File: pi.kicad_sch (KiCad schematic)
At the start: 5 parts, among them J5 2-1734839-0, J6 2-1734839-0, U15 MCP23008-E/ML

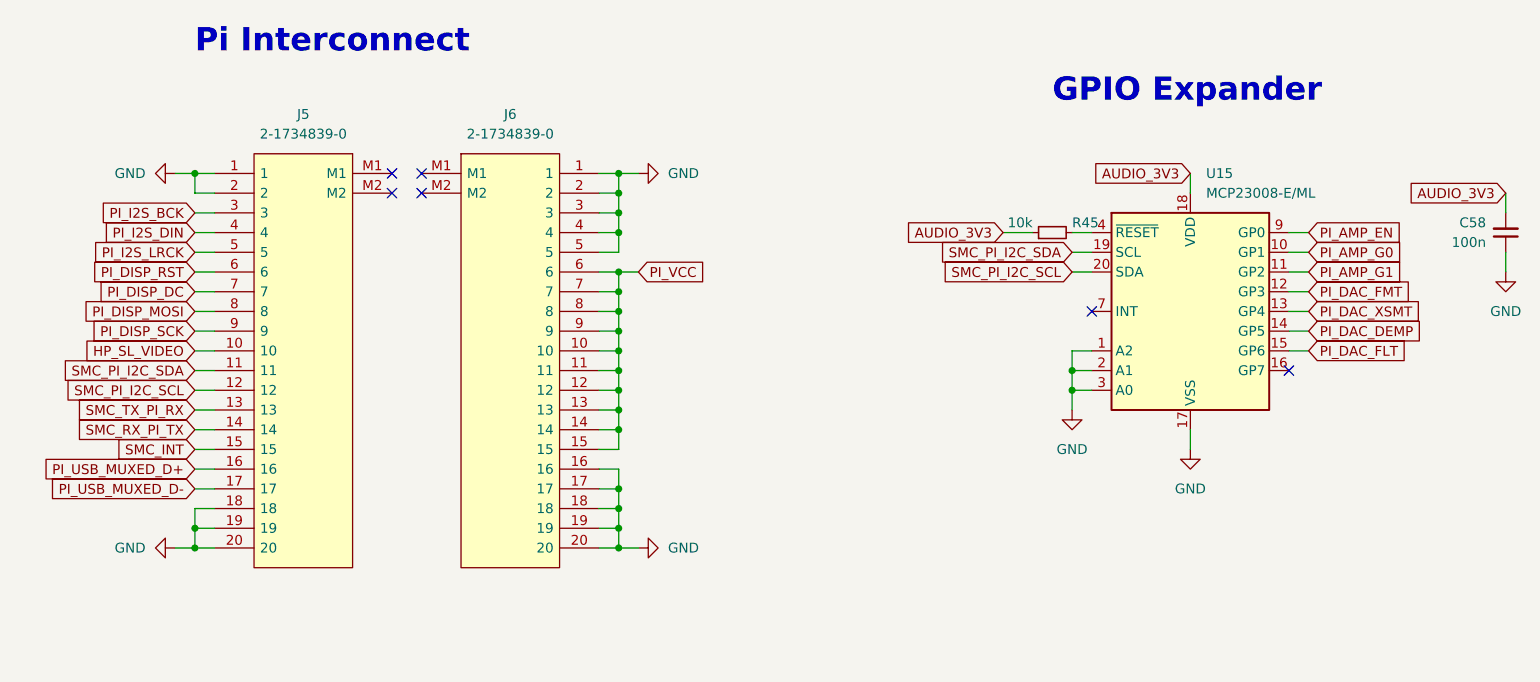
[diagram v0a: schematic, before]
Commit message: routing: begin routing
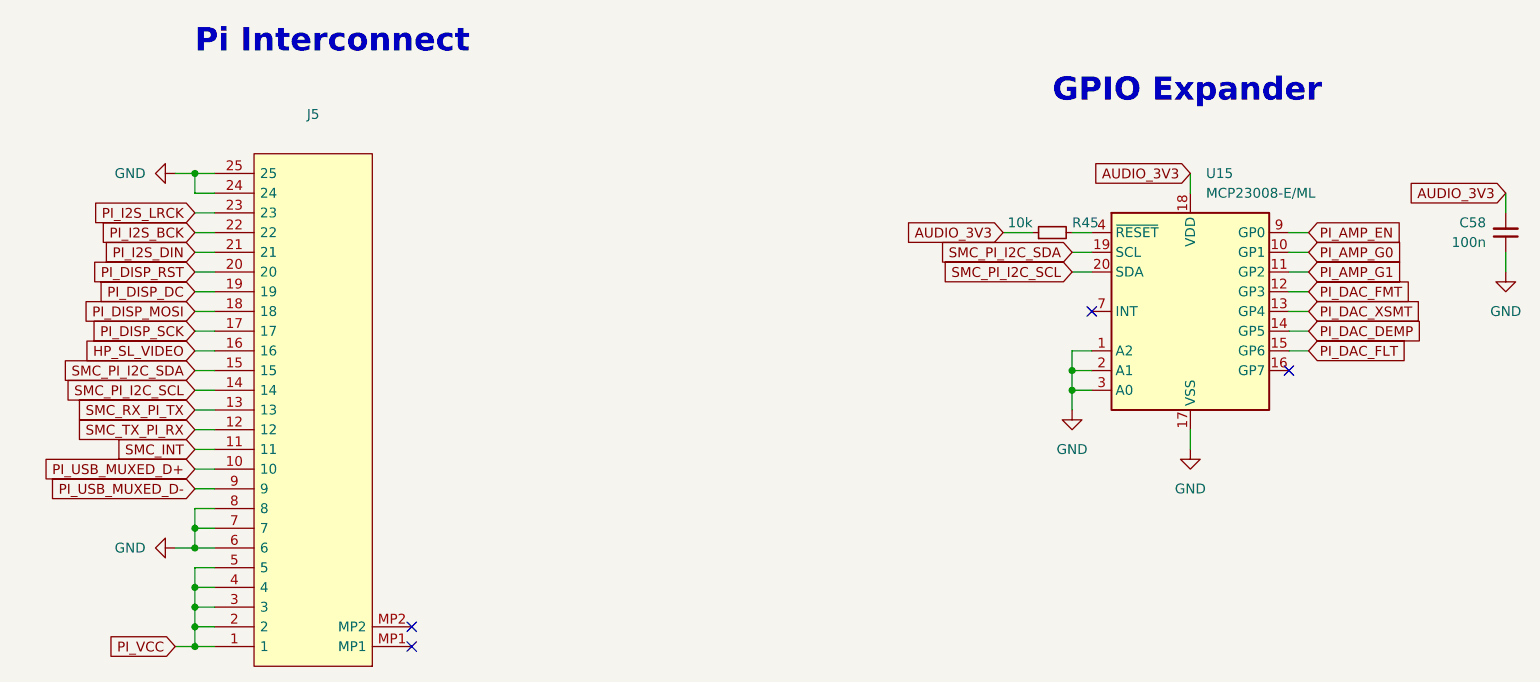
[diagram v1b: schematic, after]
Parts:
- removed J5, J6: 2-1734839-0, Gigahawk:2-1734839-0, symbol gigahawk:2-1734839-0
- added J5: (no value), symbol gigahawk:2-1734839-5
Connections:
- net GND: now also J5.24, J5.25, J5.6, J5.7, J5.8
- net HP_SL_VIDEO: now also J5.16
- net PI_DISP_DC: now also J5.19
- net PI_DISP_MOSI: now also J5.18
- net PI_DISP_RST: now also J5.20
- net PI_DISP_SCK: now also J5.17
- net PI_I2S_BCK: now also J5.22
- net PI_I2S_DIN: now also J5.21
- net PI_I2S_LRCK: now also J5.23
- net PI_USB_MUXED_D+: now also J5.10
- net PI_USB_MUXED_D-: now also J5.9
- net PI_VCC: now also J5.1, J5.2, J5.3, J5.4, J5.5
- net SMC_INT: now also J5.11
- net SMC_PI_I2C_SCL: now also J5.14
- net SMC_PI_I2C_SDA: now also J5.15
- net SMC_RX_PI_TX: now also J5.13
- net SMC_TX_PI_RX: now also J5.12
- no-connect marks 6 -> 4
